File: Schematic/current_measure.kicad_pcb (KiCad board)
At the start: 2 copper layers, 75.9 x 52.3 mm, 62 parts, among them J1 Conn_01x04_Pin, J2 Screw_Terminal_01x02, J3 Conn_01x02, J4 PowerSupply select, J5 Conn_02x03_Counter_Clockwise, J6 Conn_01x04, Q1 Si2319CDS, SW1 SW_Push, U1 6N137, U2 6N137, U3 INA186, U5 MIC5365-3.3YD5, U6 STM32G431C8Tx, U7 OPA350, U8 OPA333xxDBV, U9 OPA333xxDBV, Y1 8MHz

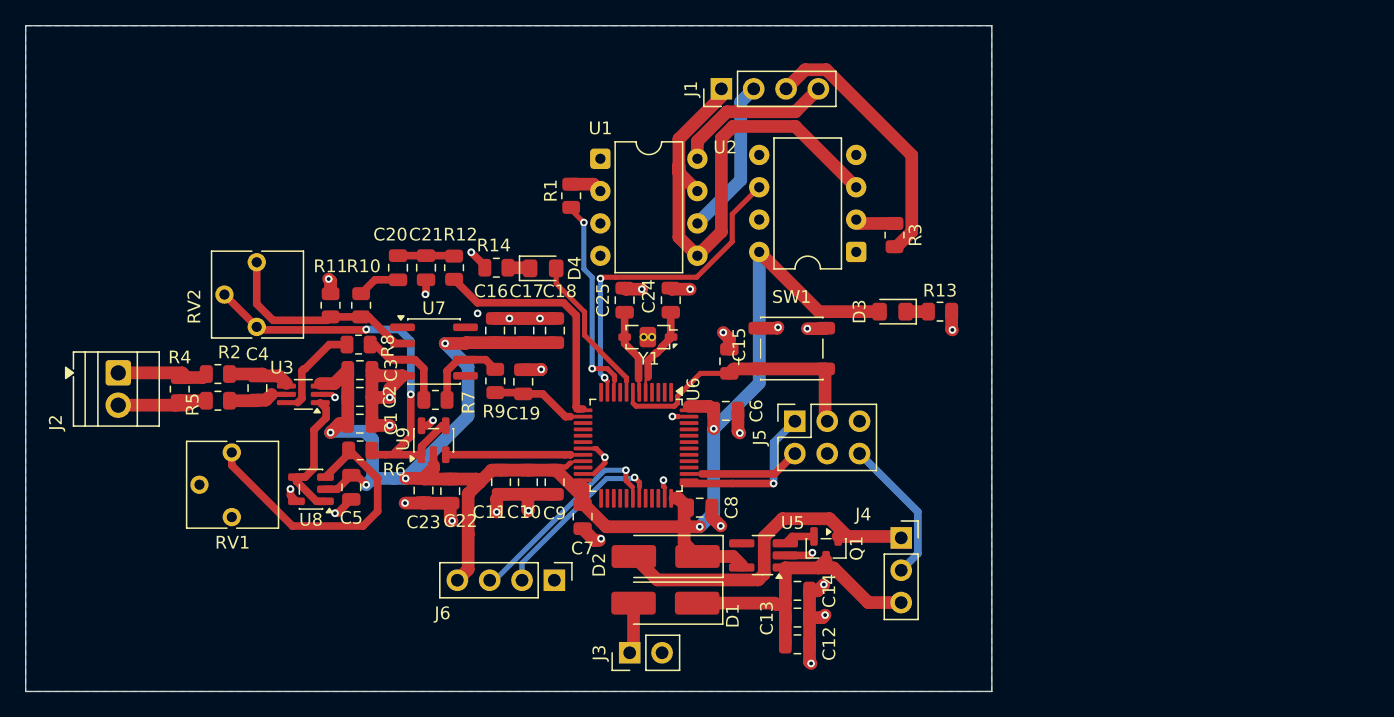
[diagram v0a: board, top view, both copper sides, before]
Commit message: improved layout
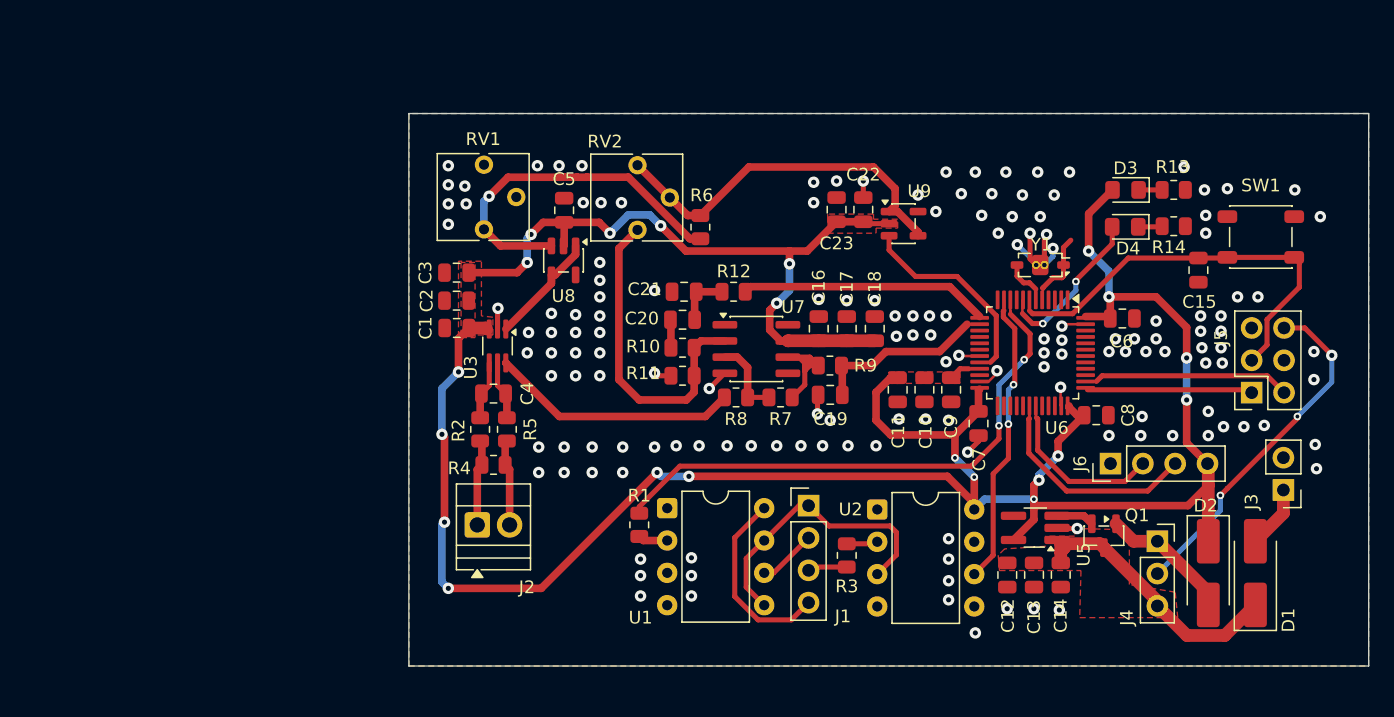
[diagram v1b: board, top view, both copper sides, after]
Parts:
- removed C24, C25: 1p, Capacitor_SMD:C_0805_2012Metric
- moved R14 53.3 mm to (189.4, 80.2), turned to 0 degrees
- moved J3 52.9 mm to (198.0, 100.9), turned to 180 degrees
- moved D1 46.4 mm to (195.8, 107.4), turned to 90 degrees
- moved D4 45.8 mm to (185.6, 80.2), turned to 180 degrees
- moved J6 44.6 mm to (184.4, 98.8), turned to 90 degrees
- moved D2 42.6 mm to (192.1, 107.4), turned to -90 degrees
- moved U9 40.6 mm to (168.2, 80.0), turned to 0 degrees
- moved C22 39.3 mm to (165.0, 78.8), turned to 90 degrees
- moved C23 39.2 mm to (162.9, 78.8), turned to 90 degrees
- moved SW1 37.9 mm to (196.2, 81.0)
- moved C15 37.5 mm to (191.3, 83.6), turned to -90 degrees
- moved J5 36.0 mm to (195.5, 93.2), turned to 180 degrees
- moved J1 33.4 mm to (160.7, 102.1), turned to 0 degrees
- moved C11 32.0 mm to (167.7, 93.0)
- moved C10 32.0 mm to (169.8, 93.0)
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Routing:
- net +3.3V: track 132.2 -> 220.9 mm, vias 6 -> 21
- net GND: track 67.9 -> 26.7 mm, vias 33 -> 153
- net MCU_TxD: track 15.7 -> 43.5 mm
- net USB_GND: track 41.3 -> 22.5 mm
- net USB_TxD: track 21.1 -> 3.11 mm
- net +3.3VP: track 26.8 -> 10.5 mm
- net Net-(J4-Pin_2): track 11.6 -> 27.9 mm, vias 0 -> 3
- net Current_measure: track 7.04 -> 19.5 mm
- net /~{RESET}: track 20.9 -> 32.5 mm
- net Net-(U7--): track 16.2 -> 25.3 mm
- net USB_RxD: track 12.6 -> 4.62 mm
- net /SWCLK: track 7.98 -> 15.5 mm
- net ADC_in: track 7.75 -> 14.5 mm
- net V_{ref}: track 11.2 -> 15.5 mm
- net Net-(U8-+): track 23.6 -> 27.8 mm, vias 0 -> 1
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- added copper zone on F.Cu, net +3.3V
- added copper zone on F.Cu, net +5V
- added copper zone on F.Cu, net GND
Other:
- board size 75.9 x 52.3 mm -> 75.4 x 43.4 mm
